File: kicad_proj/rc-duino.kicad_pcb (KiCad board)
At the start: 4 copper layers, 99.6 x 50.2 mm, 53 parts, among them J1 Conn_01x03_Male, J10 Conn_01x04_Male, J11 Conn_01x03_Male, J12 Conn_01x03_Male, J13 Conn_01x02_Male, J14 Conn_01x02_Male, J2 Conn_01x04_Male, J3 Conn_01x02_Male, J4 Conn_01x08_Male, J5 Conn_01x08_Male, J6 Conn_01x08_Male, J7 Conn_01x03_Male, J8 Conn_02x03_Odd_Even, J9 Conn_01x06_Male, U1 rc2014_Ebus-CPU, U2 ATMEGA2560-16AUR, U3 74HCT595D, U4 SN74LVC1G374DCKR, U5 74HCT688, U6 74LVC1G3157, U7 74LVC1G3157, U8 74HCT688, U9 SN74LVC1G08DCKR, Y1 16Mhz Crystal

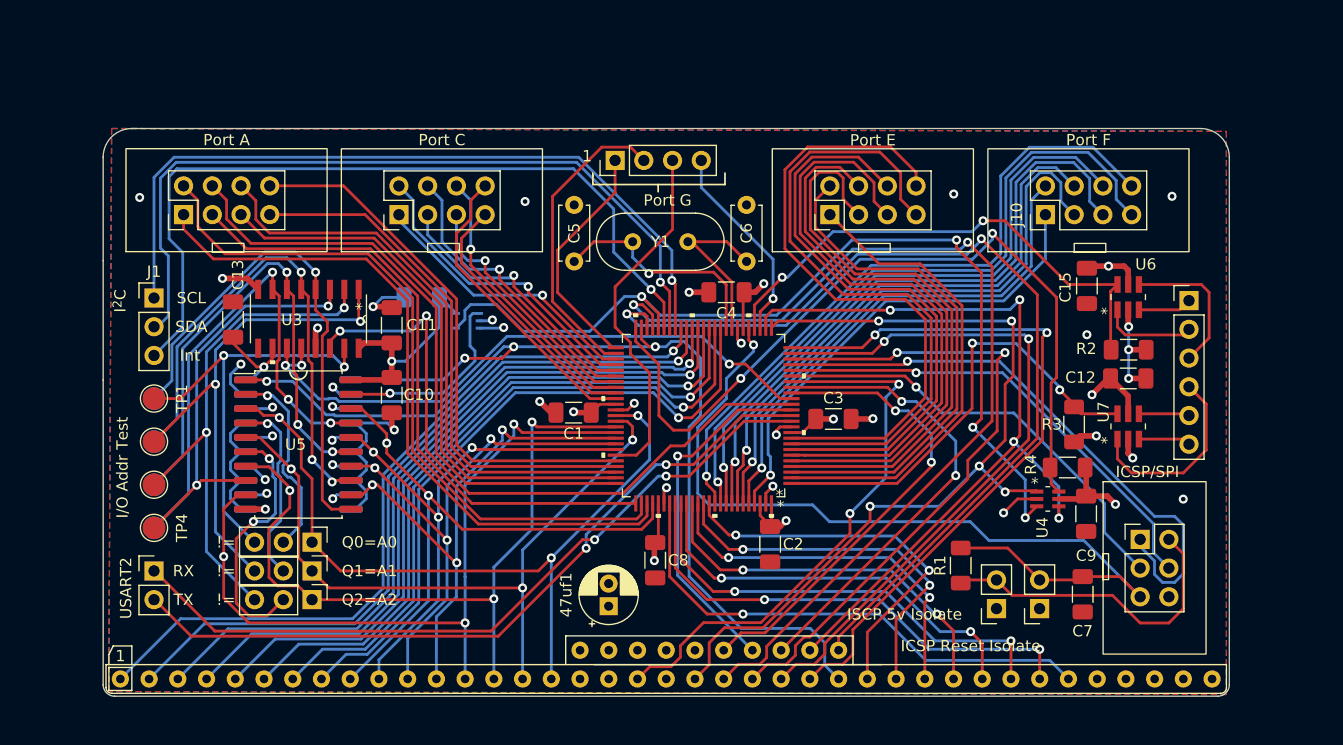
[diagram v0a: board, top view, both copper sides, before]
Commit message: major rework
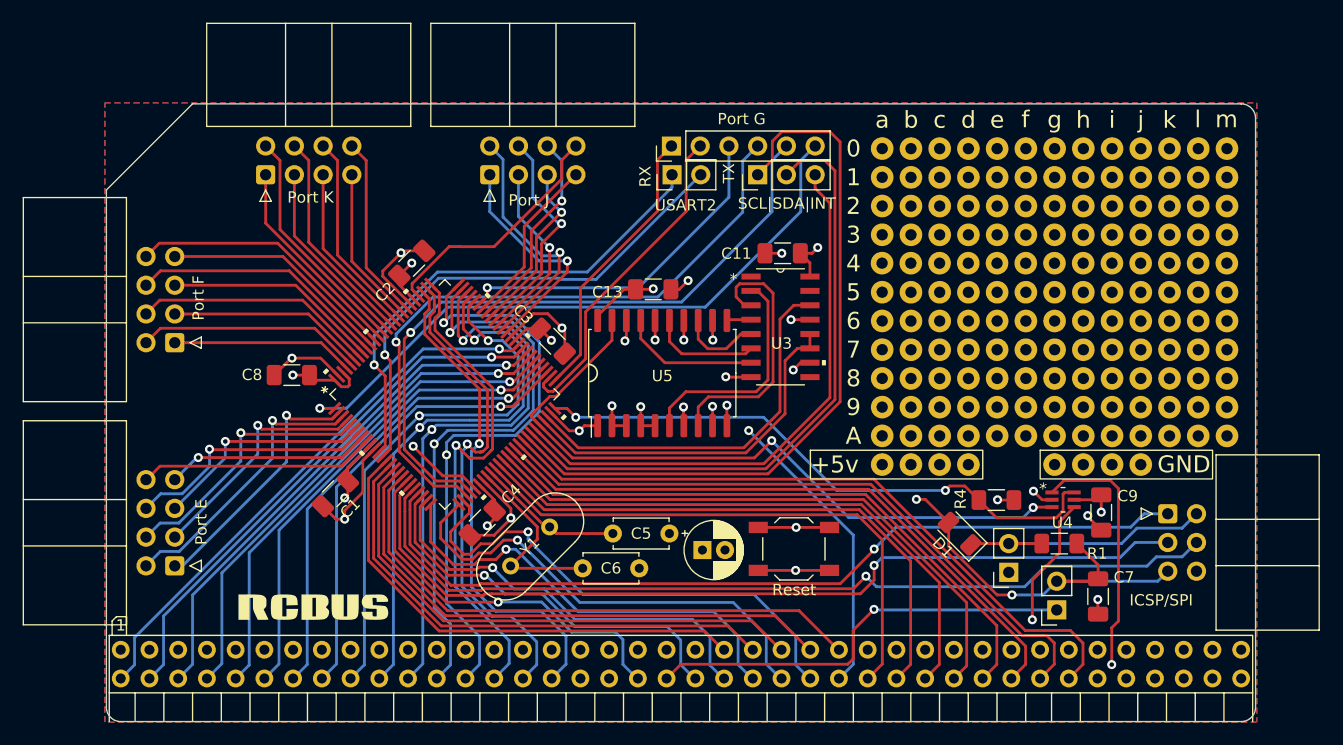
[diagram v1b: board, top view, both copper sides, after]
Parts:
- removed C10, C12, C14, C15: .1uf, Capacitor_SMD:C_1206_3216Metric_Pad1.33x1.80mm_HandSolder
- removed J11, J12: Conn_01x03_Male, Connector_PinHeader_2.54mm:PinHeader_1x03_P2.54mm_Vertical
- removed J9: Conn_01x06_Male, Connector_PinHeader_2.54mm:PinHeader_1x06_P2.54mm_Vertical
- removed R2, R3: 10k, Resistor_SMD:R_1206_3216Metric_Pad1.30x1.75mm_HandSolder
- removed TP1, TP10, TP2, TP3, TP4, TP5, TP6, TP9: TestPoint, TestPoint:TestPoint_Pad_D2.0mm
- removed U6, U7: 74LVC1G3157, lib-rc-duino:SN74LVC1G3157DBVR
- removed U8: 74HCT688, Package_SO:SOIC-20W_7.5x12.8mm_P1.27mm
- removed U9: SN74LVC1G08DCKR, lib-rc-duino:DCK5-L
- added D1: D, Diode_SMD:D_1206_3216Metric, F.Cu at (134.2, 74.9)
- added H2: RCBus Logo, lib-rc-duino:RCBUS, F.Cu at (77.3, 81.4)
- added Reset: SW_Push, Button_Switch_SMD:SW_SPST_TL3342, F.Cu at (119.5, 76.2)
- H1: value MountingHole -> AVRC-Logo
- J10, J4, J5, J6: footprint lib-rc-duino:Boxed_PinHeader_2x04_P2.54mm_Vertical -> Connector_IDC:IDC-Header_2x04_P2.54mm_Horizontal
- J2: value Conn_01x04_Male -> Conn_01x06_Male; footprint Connector_PinHeader_2.54mm:PinHeader_1x04_P2.54mm_Vertical -> Connector_PinHeader_2.54mm:PinHeader_1x06_P2.54mm_Vertical
- J7: value Conn_01x03_Male -> proto_area_power_gnd; footprint Connector_PinHeader_2.54mm:PinHeader_1x03_P2.54mm_Vertical -> lib-rc-duino:protoarea
- J8: footprint lib-rc-duino:Boxed_PinHeader_2x03_P2.54mm_Vertical -> Connector_IDC:IDC-Header_2x03_P2.54mm_Horizontal
- U1: value rc2014_Ebus-CPU -> RCBus; footprint lib-rc-duino:Header_busBackPlane -> lib-rc-duino:RCBus
- moved J10 77.8 mm to (64.8, 58.0), turned to 180 degrees
- moved J6 65.7 mm to (64.8, 77.7), turned to 180 degrees
- moved J7 61.3 mm to (127.3, 40.8), turned to 0 degrees
- moved J3 57.7 mm to (108.7, 43.1), turned to 90 degrees
- moved U1 56.9 mm to (63.8, 55.9), turned to 0 degrees
- moved J1 54.5 mm to (116.3, 43.1), turned to 90 degrees
- moved U3 41.7 mm to (118.3, 56.6), turned to 0 degrees
- moved C2 40.3 mm to (85.7, 51.0), turned to 45 degrees
- moved C13 37.2 mm to (107.1, 53.3), turned to 0 degrees
- moved C8 36.1 mm to (75.1, 60.8), turned to 0 degrees
- moved C11 35.1 mm to (118.5, 50.1), turned to 180 degrees
- moved U5 32.8 mm to (107.9, 60.7), turned to 90 degrees
- moved C6 30.8 mm to (100.8, 77.9), turned to 0 degrees
- moved C4 29.7 mm to (91.9, 73.9), turned to -135 degrees
- moved J4 27.3 mm to (92.6, 43.1)
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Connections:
- J4 pad 1: /pa0 -> /pj0
- J4 pad 2: /pa1 -> /pj1
- J4 pad 3: /pa2 -> /pj2
- J4 pad 4: /pa3 -> /pj3
- J4 pad 5: /pa4 -> /pj4
- J4 pad 6: /pa5 -> /pj5
- J4 pad 7: /pa6 -> /pj6
- J4 pad 8: /pa7 -> /pj7
- J5 pad 1: /pc0 -> /pk0
- J5 pad 2: /pc1 -> /pk1
- J5 pad 3: /pc2 -> /pk2
- J5 pad 4: /pc3 -> /pk3
- J5 pad 5: /pc4 -> /pk4
- J5 pad 6: /pc5 -> /pk5
- J5 pad 7: /pc6 -> /pk6
- J5 pad 8: /pc7 -> /pk7
- J7 pad 1: A0 -> VCC
- J7 pad 2: /jmpA0 -> prog_gnd
- U2 pad 1: man_clock_toggle -> /pg5
- U2 pad 14: Halt -> BusAck
- U2 pad 15: port_sr_data -> Halt
- U2 pad 16: port_sr_clk -> BusRQ
- U2 pad 17: BusAck -> ~{WAIT}
- U2 pad 18: BusRQ -> NMI
- U2 pad 23: MREQ -> CLK
- U2 pad 24: WR -> INT
- U2 pad 25: RD -> MREQ
- U2 pad 26: CLK -> WR
- U2 pad 27: ~{WAIT} -> RD
- U2 pad 29: man_clock_en -> /pg4
- U2 pad 35: A8 -> D0
- U2 pad 36: A9 -> D1
- U2 pad 37: Aa -> D2
- U2 pad 38: Ab -> D3
- U2 pad 39: Ac -> D4
- U2 pad 40: Ad -> D5
- U2 pad 41: Ae -> D6
- U2 pad 42: Af -> D7
- U2 pad 47: INT -> port_sr_clk
- U2 pad 48: NMI -> port_sr_data
- U2 pad 53: /pc0 -> A8
- U2 pad 54: /pc1 -> A9
- U2 pad 55: /pc2 -> Aa
- U2 pad 56: /pc3 -> Ab
- U2 pad 57: /pc4 -> Ac
- U2 pad 58: /pc5 -> Ad
- U2 pad 59: /pc6 -> Ae
- U2 pad 60: /pc7 -> Af
- U2 pad 63: A0 -> /pj0
- U2 pad 64: A1 -> /pj1
- U2 pad 65: A2 -> /pj2
- U2 pad 66: A3 -> /pj3
- U2 pad 67: A4 -> /pj4
- U2 pad 68: A5 -> /pj5
- U2 pad 69: A6 -> /pj6
- U2 pad 71: /pa7 -> A7
- U2 pad 72: /pa6 -> A6
- U2 pad 73: /pa5 -> A5
- U2 pad 74: /pa4 -> A4
- U2 pad 75: /pa3 -> A3
- U2 pad 76: /pa2 -> A2
- U2 pad 77: /pa1 -> A1
- U2 pad 78: /pa0 -> A0
- U2 pad 79: A7 -> /pj7
- U2 pad 82: D7 -> /pk7
- U2 pad 83: D6 -> /pk6
- U2 pad 84: D5 -> /pk5
- U2 pad 85: D4 -> /pk4
- U2 pad 86: D3 -> /pk3
- U2 pad 87: D2 -> /pk2
- U2 pad 88: D1 -> /pk1
- U2 pad 89: D0 -> /pk0
- U3 pad 1: /Q1 -> unconnected-(U3-Pad1)
- U3 pad 15: /Q0 -> unconnected-(U3-Pad15)
- U3 pad 2: /Q2 -> Net-(U3-Pad2)
- U5 pad 19: Net-(U5-Pad19) -> ~{portIOrequest}
- U5 pad 2: /jmpA0 -> A0
- U5 pad 4: /jmpA1 -> A1
- U5 pad 6: /jmpA2 -> Net-(U3-Pad2)
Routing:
- net /pa1: track 63.1 -> 0.00 mm
- net /pa0: track 62.4 -> 0.00 mm
- net /pg4: track 0.00 -> 60.7 mm, vias 0 -> 1
- net /pg5: track 0.00 -> 57.4 mm, vias 0 -> 1
- net /pa2: track 55.9 -> 0.00 mm
- net /pa3: track 55.1 -> 0.00 mm
- net ~{IORQ}: track 100.8 -> 46.6 mm, vias 4 -> 2
- net /pa5: track 52.1 -> 0.00 mm
- net /pa4: track 50.3 -> 0.00 mm
- net INT: track 86.6 -> 37.3 mm, vias 2 -> 1
- net /pa7: track 48.2 -> 0.00 mm
- net /pa6: track 47.4 -> 0.00 mm
- net /Q2: track 45.7 -> 0.00 mm, vias 2 -> 0
- net man_clock_en: track 45.6 -> 0.00 mm, vias 2 -> 0
- net /Q1: track 45.4 -> 0.00 mm, vias 2 -> 0
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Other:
- board size 99.6 x 50.2 mm -> 101.6 x 54.6 mm
- board text added: "INT|SDA|SCL"
- board text added: "Port J"
- board text added: "Port K"
- board text added: "SCL|SDA|INT"
- board text added: "v6"
- board text removed: "!="
- board text removed: "1"
- board text removed: "C"
- board text removed: "Clock Ctrl"
- board text removed: "Dflt"
- board text removed: "I/O Addr Test"
- board text removed: "ICSP Reset Isolate"
- board text removed: "ISCP 5v Isolate"
- board text removed: "I^{2}C"
- board text removed: "Int"
- board text removed: "Man"
- board text removed: "NC"
- board text removed: "NO"
- board text removed: "Port A"
- board text removed: "Port C"
- board text removed: "Q0=A0"
- board text removed: "Q1=A1"
- board text removed: "Q2=A2"
- board text removed: "Rtn"
- board text removed: "SCL"
- board text removed: "SDA"
- board text removed: "v5"
